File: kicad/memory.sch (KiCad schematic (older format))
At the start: 33 parts, among them SW3 SW_DIP_x08, SW5 SW_DIP_x04, U32 74LS04, U35 74LS173, U36 74LS157, U37 74LS157, U38 74LS189, U39 74LS189, U40 74LS157, U41 74LS04, U42 74LS00, U43 74LS245, U44 74LS157

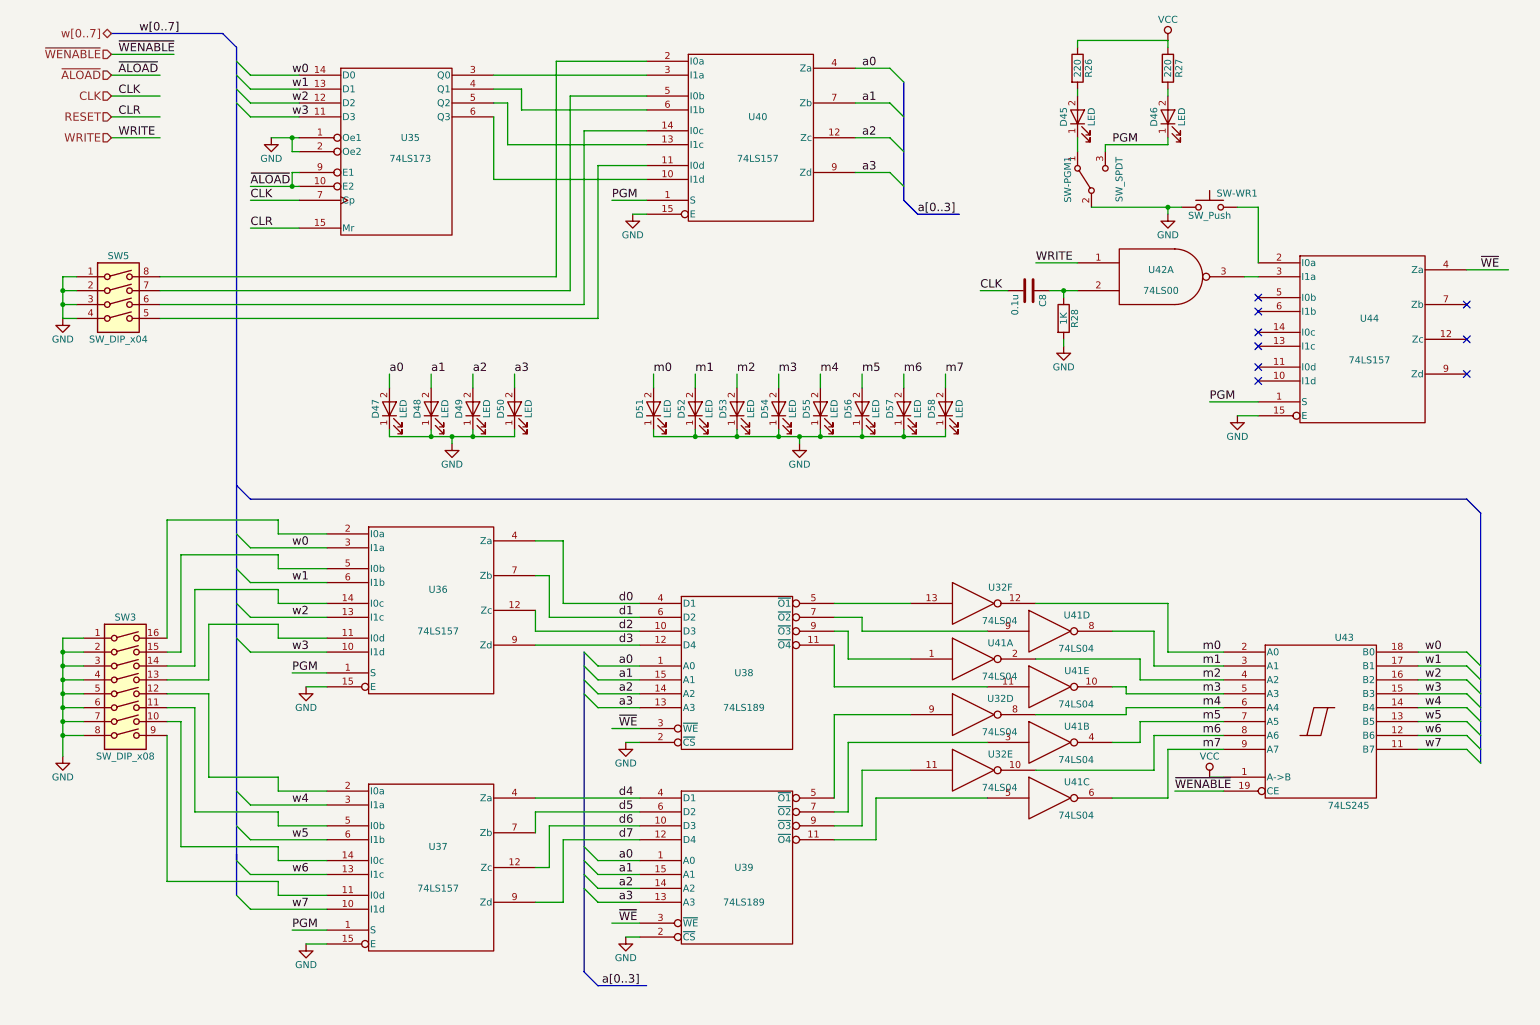
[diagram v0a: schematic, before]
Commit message: Update to current kicad libraries
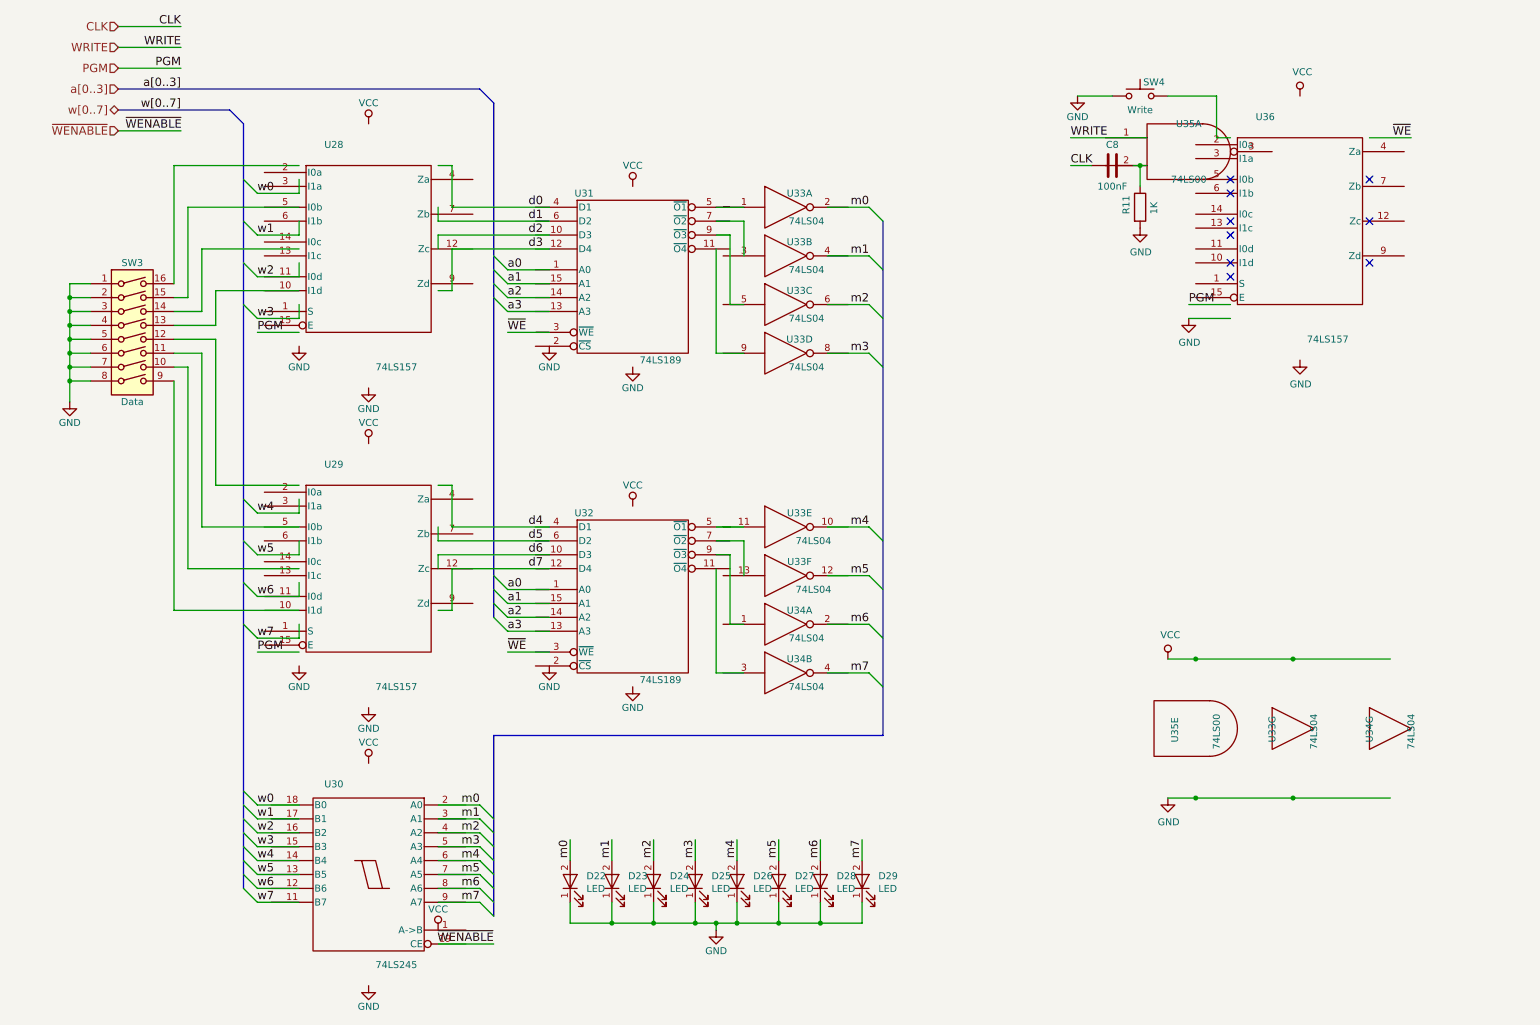
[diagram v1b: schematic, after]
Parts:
- removed C8: 0.1u, Capacitors_THT:C_Disc_D6_P5, symbol C
- removed D45, D46, D47, D48, D49, D50, D51, D52, D53, D54, D55, D56, D57, D58: LED, LEDs:LED-5MM, symbol LED
- removed R26, R27: 220, Resistors_THT:Resistor_Horizontal_RM7mm, symbol R
- removed R28: 1K, Resistors_THT:Resistor_Horizontal_RM7mm, symbol R
- removed SW-PGM1: SW_SPDT, Buttons_Switches_THT:SW_Micro_SPST, symbol SW_SPDT
- removed SW-WR1: SW_Push, Buttons_Switches_THT:SW_PUSH_6mm_h9.5mm, symbol SW_Push
- removed SW3: SW_DIP_x08, Buttons_Switches_THT:SW_DIP_x8_Slide, symbol SW_DIP_x08
- removed SW5: SW_DIP_x04, Buttons_Switches_THT:SW_DIP_x4_Slide, symbol SW_DIP_x04
- removed U32, U41: 74LS04, Housings_DIP:DIP-14_W7.62mm_LongPads, symbol 74LS04
- removed U35: 74LS173, Housings_DIP:DIP-16_W7.62mm_LongPads, symbol 74LS173
- removed U36, U37, U40, U44: 74LS157, Housings_DIP:DIP-16_W7.62mm_LongPads, symbol 74LS157
- removed U38, U39: 74LS189, Housings_DIP:DIP-16_W7.62mm_LongPads, symbol 74LS189
- removed U42: 74LS00, Housings_DIP:DIP-14_W7.62mm_LongPads, symbol 74LS00
- removed U43: 74LS245, Housings_DIP:DIP-20_W7.62mm_LongPads, symbol 74LS245
- added C8: 100nF, symbol Device:C
- added D22, D23, D24, D25, D26, D27, D28, D29: LED, symbol Device:LED
- added R11: 1K, symbol Device:R
- added SW3: Data, symbol Switch:SW_DIP_x08
- added SW4: Write, symbol Switch:SW_Push
- added U28, U29, U36: 74LS157, symbol 74xx:74LS157
- added U30: 74LS245, symbol 74xx:74LS245
- added U31, U32: 74LS189, symbol sap-be:74LS189
- added U33, U34: 74LS04, symbol 74xx:74LS04
- added U35: 74LS00, symbol 74xx:74LS00
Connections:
- net labels removed: CLR, RESET, ~ALOAD
- wire segments 242 -> 174
